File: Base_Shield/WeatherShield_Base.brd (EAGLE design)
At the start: 58.4 x 67.3 mm, 68 parts, among them Q1 BSS138, Q2 BSS138, U1 DS3231SN, U2 LT3652, U3 TMP100MDBVREP, U4 ADS1015IDGST

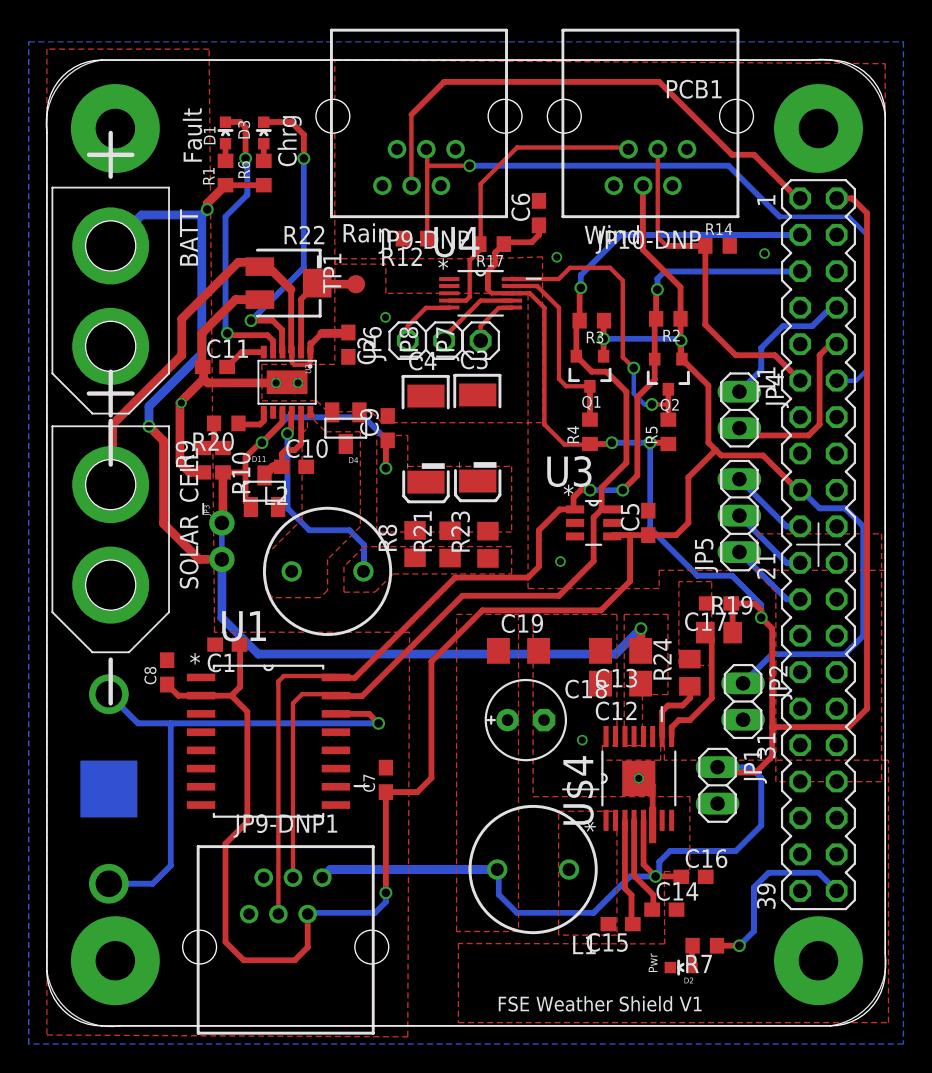
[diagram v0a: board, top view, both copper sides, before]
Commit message: WeatherShield_v1
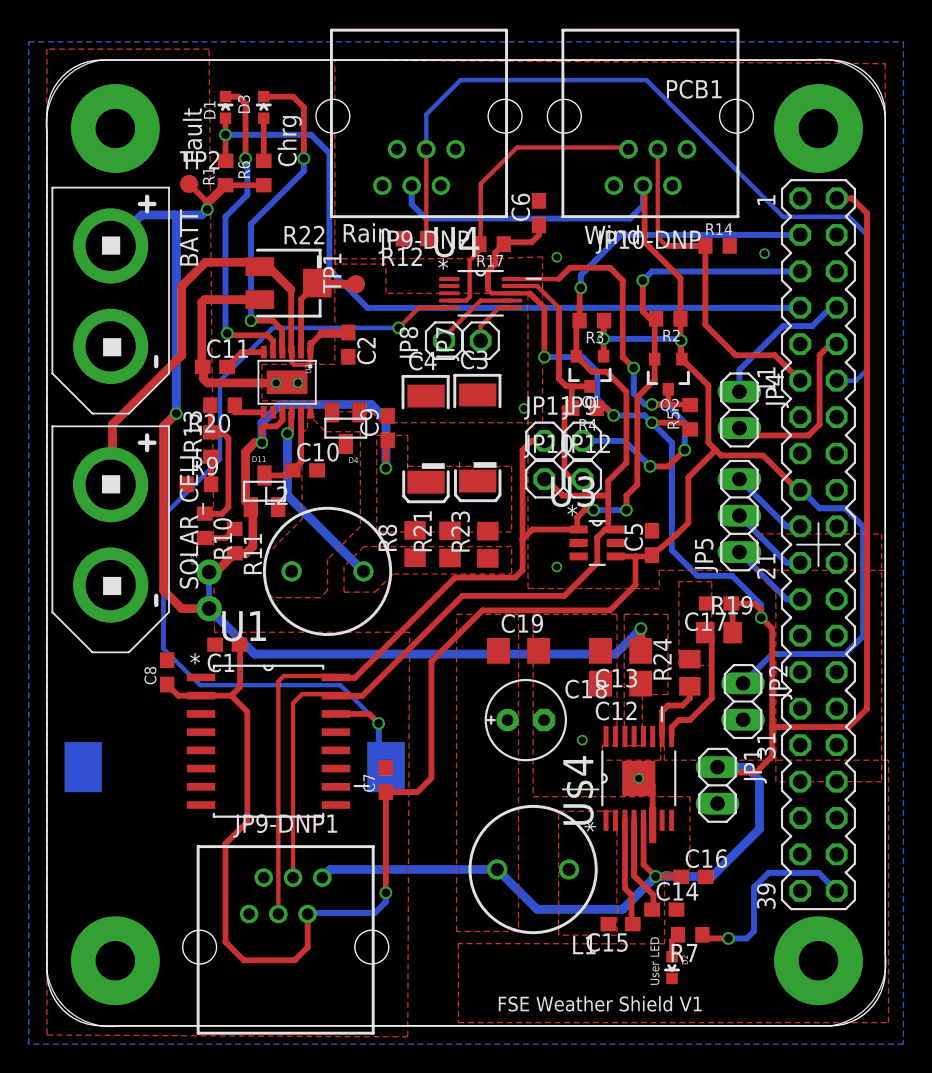
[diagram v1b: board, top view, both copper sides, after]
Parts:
- removed G1: 3V, battery:CELL_RETAINER_11.6MM
- removed JP6: (no value), pinhead:1X01
- added JP10, JP11, JP12, JP9: (no value), pinhead:1X01
- added R11, R13: 0, rcl:R0603
- added TP2: SET, testpad:B1,27
- added U$1: BATTERIE_HALTER_CR1225, FSEWeatherShield:BATTERIE_HALTER_CR1225
- moved R10 4.75 mm to (12.1, 35.9)
- moved JP3 3.54 mm to (12.4, 31.4)
- moved R5 1.83 mm to (46.0, 43.4)
- moved D1 1.78 mm to (13.6, 65.0)
- moved D3 1.78 mm to (16.3, 65.0)
- moved R9 1.70 mm to (11.7, 38.8), turned to 0 degrees
- moved R4 1.69 mm to (38.6, 44.1), turned to 180 degrees
- moved C5 1.42 mm to (43.3, 34.7)
- moved U3 1.42 mm to (39.5, 34.7)
- moved R20 1.30 mm to (13.4, 44.3)
- moved R7 1.27 mm to (46.0, 7.37)
- moved C10 0.80 mm to (19.1, 39.7)
- moved D2 0.63 mm to (44.7, 5.08), turned to 180 degrees
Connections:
- removed net N$14: JP6.1, U4.5
- removed net N$6: G1.P+@1, G1.P+@2, U1.14
- new net FAULT_PIN: D1.A, PCB1.7, R1.2
- new net N$1: R13.1, R9.2
- new net N$2: R10.2, R11.1
- new net RTC_BATT: U$1.P, U1.14, U4.5
- net FB: now also R13.2; no longer R9.2
- net GND: now also U$1.N; no longer G1.N-
- net HV_SCL: now also JP9.1
- net HV_SDA: now also JP12.1
- net N$16: now also R11.2; no longer R10.2
- net N$3: now also PCB1.16; no longer D1.A, R1.2
- net SCL: now also JP11.1
- net SDA: now also JP10.1
- net V_BATT: now also TP2.TP
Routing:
- net RTC_BATT: track 0.00 -> 62.2 mm, vias 0 -> 2
- net FAULT_PIN: track 0.00 -> 52.9 mm, vias 0 -> 1
- net N$6: track 37.6 -> 0.00 mm, vias 1 -> 0
- net 3.3V: track 187.9 -> 170.4 mm
- net HV_SCL: track 21.5 -> 35.0 mm, vias 2 -> 4
- net SCL: track 73.9 -> 84.4 mm
- net GND: track 30.4 -> 23.2 mm, vias 9 -> 8
- net HV_SDA: track 13.6 -> 20.5 mm
- net FB: track 3.18 -> 9.95 mm
- net RAIN: track 50.7 -> 56.7 mm, vias 1 -> 0
- net SDA: track 77.6 -> 83.0 mm
- net N$16: track 27.1 -> 31.7 mm
- net N$14: track 4.46 -> 0.00 mm
- net N$2: track 0.00 -> 2.35 mm
- net N$1: track 0.00 -> 1.92 mm
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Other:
- board text added: "User LED"
- board text removed: "Pwr"
